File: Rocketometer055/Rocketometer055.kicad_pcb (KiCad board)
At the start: 2 copper layers, 55.9 x 22.9 mm, 58 parts, among them J102 Micro_SD_Card_Det_Hirose_DM3AT, J601 USB_MICROB, J801 JST 2mm, Q650 PMOS, U101 LPC2148, U201 BME280, U301 BNO085, U401 ADXL375, U501 FGPMMOPA6H, U599 FGPMMOPA6H, U701 3.3V, U801 MCP73831, Y101 12MHz, Y301 32kiHz

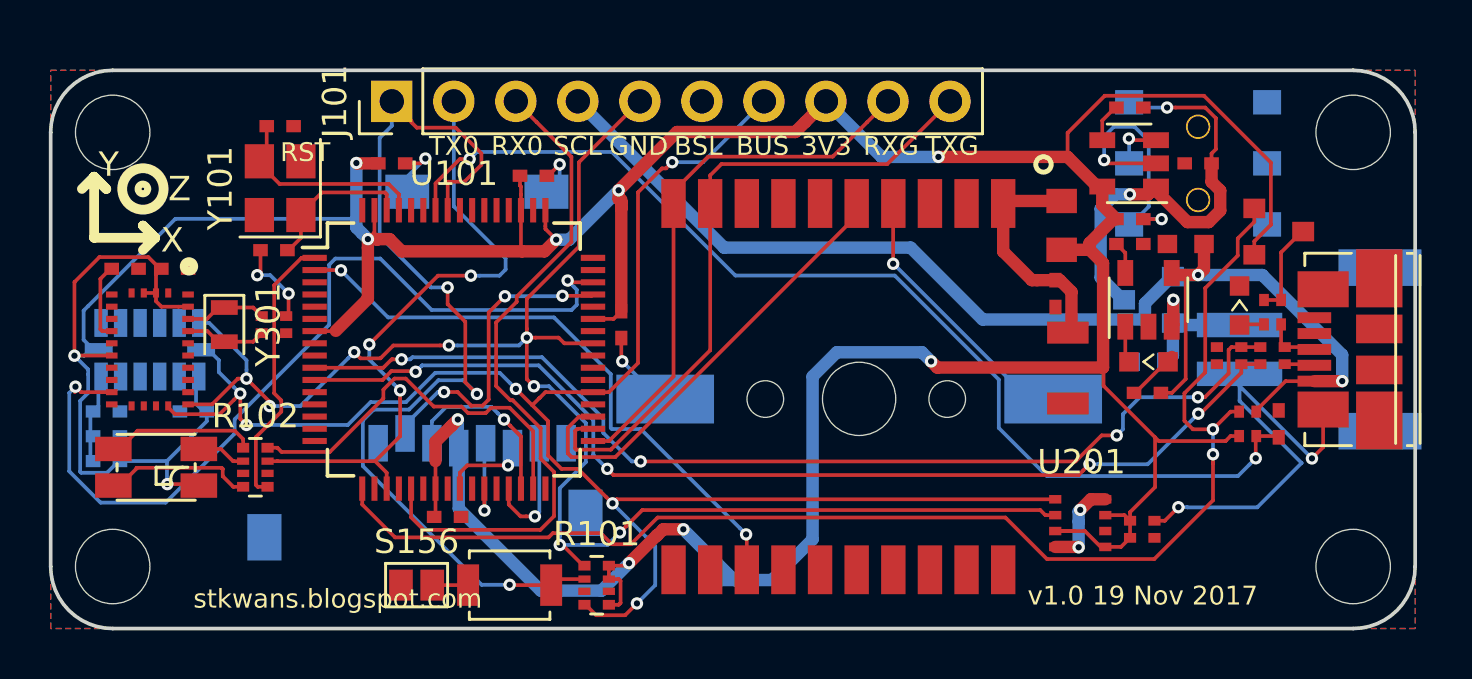
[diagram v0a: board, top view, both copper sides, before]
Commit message: Working on Rocketometer055
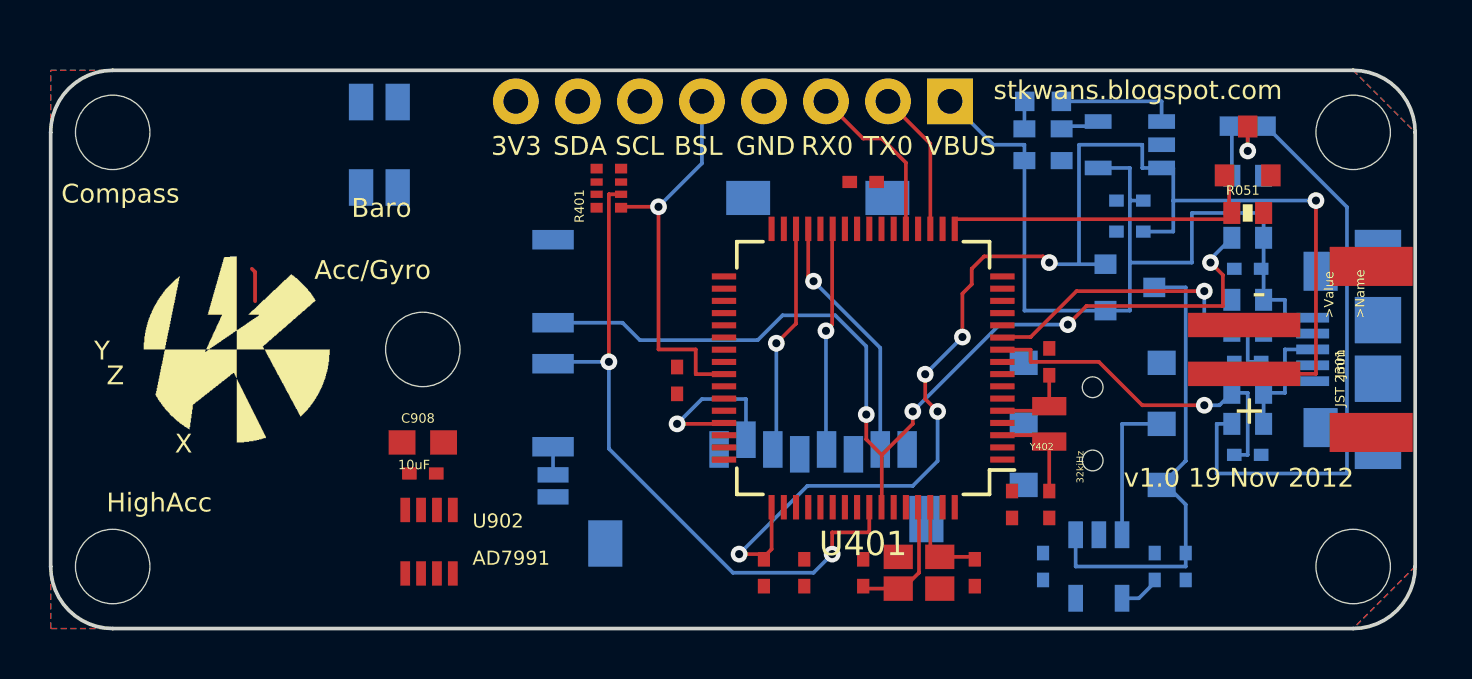
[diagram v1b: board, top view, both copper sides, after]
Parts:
- removed B504: Coin_Cell, KwanSystems:CR1220-2
- removed C123, C406, C704: 1uF, KwanSystems:SMD_0402
- removed C143, C151, C163, C401, C501, C714: 100nF, KwanSystems:SMD_0402
- removed C161, C162: 33pF, KwanSystems:SMD_0402
- removed C206: 100nF, KwanSystems:R_Array_Convex_2x0402
- removed C303, C309: 0.1uF, KwanSystems:SMD_0402
- removed C326, C623: 22pF, KwanSystems:R_Array_Convex_2x0402
- removed C503: 10uF, KwanSystems:SMD_1206
- removed C715: 4.7nF, KwanSystems:SMD_0402
- removed C802, C803: 4.7uF, KwanSystems:SMD_0603
- removed D101: HSMF-C118, KwanSystems:HSMF-C118
- removed D650: BLUE, KwanSystems:D_0603
- removed D801: YELLOW, KwanSystems:D_0603
- removed D802: DCC, KwanSystems:SOT-23
- removed J101: ~, Pin_Headers:Pin_Header_Straight_1x10_Pitch2.54mm
- removed J102: Micro_SD_Card_Det_Hirose_DM3AT, KwanSystems:MICROSD-SOCKET-PP
- removed J601: USB_MICROB, KwanSystems:USB_Micro-B_Molex_47346-0001
- removed J801: JST 2mm, KwanSystems:SPARKFUN_JST_POWER
- removed L501: Ferrite, KwanSystems:SMD_0805
- removed Q650: PMOS, KwanSystems:SOT-23
- removed R101: 10k, KwanSystems:R_Array_Convex_4x0402
- removed R102: 1.5k, KwanSystems:R_Array_Convex_4x0402
- removed R406: 100, KwanSystems:SMD_0402
- removed R611: 22k, KwanSystems:SMD_0402
- removed R623: 33, KwanSystems:R_Array_Convex_2x0402
- removed R650: 1.5k, KwanSystems:R_Array_Convex_2x0402
- removed R651: 10k, KwanSystems:R_Array_Convex_2x0402
- removed R801: 10k, KwanSystems:SMD_0402
- removed R804: 1.5k, KwanSystems:SMD_0402
- removed S156: SOLDERJUMPERNO, Connectors:GS2
- removed S157: SPST, KwanSystems:SW_SPST_B3U-1000P
- removed S701: SPDT, KwanSystems:SWITCH_DPDT_AZY0202
- removed U101: LPC2148, Housings_QFP:LQFP-64_10x10mm_Pitch0.5mm
- removed U501: FGPMMOPA6H, KwanSystems:FGPMMOPA6H
- removed U599: FGPMMOPA6H, KwanSystems:Axis
- removed U701: 3.3V, TO_SOT_Packages_SMD:SOT-23-5
- removed U801: MCP73831, TO_SOT_Packages_SMD:SOT-23-5
- removed Y101: 12MHz, Crystals:Crystal_SMD_Abracon_ABM8G-4pin_3.2x2.5mm
- removed Y301: 32kiHz, Crystals:Crystal_SMD_2012-2pin_2.0x1.2mm
- added C010: 1uF, KwanSystems:SMD_0402, B.Cu at (176.0, 86.9)
- added C020: 22pF, KwanSystems:SMD_0402, B.Cu at (176.0, 90.7)
- added C030: 22pF, KwanSystems:SMD_0402, B.Cu at (176.0, 94.5)
- added C204: 1uF, KwanSystems:SMD_0402, B.Cu at (173.5, 99.1)
- added C214: 100nF, KwanSystems:SMD_0402, B.Cu at (172.2, 99.1)
- added C215: 4.7nF, KwanSystems:SMD_0402, B.Cu at (167.6, 99.1)
- added C301: 4.7uF, KwanSystems:SMD_0402, B.Cu at (171.2, 85.3)
- added C302: 4.7uF, KwanSystems:SMD_0402, B.Cu at (171.2, 84.1)
- added C403: 18pF, KwanSystems:SMD_0402, F.Cu at (167.9, 96.5)
- added C423: 1uF, KwanSystems:SMD_0402, F.Cu at (160.3, 83.3)
- added C443: 100nF, KwanSystems:SMD_0402, F.Cu at (152.7, 91.4)
- added C449: 100nF, KwanSystems:SMD_0402, F.Cu at (156.2, 99.3)
- added C451: 100nF, KwanSystems:SMD_0402, F.Cu at (157.9, 99.3)
- added C461: 33pF, KwanSystems:SMD_0402, F.Cu at (160.3, 99.3)
- added C462: 33pF, KwanSystems:SMD_0402, F.Cu at (164.8, 99.3)
- added C463: 100nF, KwanSystems:SMD_0402, F.Cu at (166.4, 96.5)
- added C907: 100nF, KwanSystems:SMD_0402, F.Cu at (142.2, 95.2)
- added C908: 10uF, 0603-CAP, F.Cu at (142.2, 94.0)
- added D050: BLUE, LED-0603, B.Cu at (176.0, 81.0)
- added D301: YELLOW, LED-0603, B.Cu at (167.6, 80.0)
- added D302: DCC, KwanSystems:SOT-23, B.Cu at (171.2, 87.6)
- added D401: HSMF-C118, HSMF-C118, B.Cu at (140.5, 81.8)
- added J001: USB_MICROB, UB-MC5BR3-SD204-4S, B.Cu at (181.4, 90.2)
- added J301: JST 2mm, JST-2-SMD, F.Cu at (179.6, 90.2)
- added J401: M07, 1X08, F.Cu at (163.8, 80.0)
- added J701: Micro_SD_Card_Det_Hirose_DM3AT, MICROSD-SOCKET-PP, B.Cu at (163.3, 83.6)
- added JP3: STAND-OFFTIGHT, STAND-OFF-TIGHT, F.Cu at (142.2, 90.2)
- added Q050: PMOS, KwanSystems:SOT-23, F.Cu at (176.0, 82.0)
- added R010: 10k, 0402-RES, B.Cu at (176.0, 85.6)
- added R011: 100k, 0402-RES, B.Cu at (176.0, 88.1)
- added R020: 33, 0402-RES, B.Cu at (176.0, 89.4)
- added R030: 33, 0402-RES, B.Cu at (176.0, 91.9)
- added R031: 1.5k, 0402-RES, B.Cu at (176.0, 93.2)
- added R050: 1.5k, 0402-RES, B.Cu at (176.0, 83.1)
- added R051: 10k, 0402-RES, F.Cu at (176.0, 84.6)
- added R301: 10k, 0402-RES, B.Cu at (168.4, 81.8)
- added R302: 1.5k, 0402-RES, B.Cu at (166.9, 81.8)
- added R401: 10k, CRA04, F.Cu at (149.9, 83.6)
- added S201: SPDT, AYZ0202, B.Cu at (169.7, 93.2)
- added S456: SOLDERJUMPERNO, SJ_2S-NO, B.Cu at (147.6, 95.8)
- added S457: SPST, B3U-1000P, B.Cu at (147.6, 92.5)
- added S458: B3U-1000P, B3U-1000P, B.Cu at (147.6, 87.4)
- added U$1: , KWAN_ACC, F.Cu at (134.6, 90.2)
- added U$4: , AXES, F.Cu at (128.3, 94.0)
- added U$5: , KWAN_ACC, B.Cu at (134.6, 90.2)
- added U$6: , OSHW_ACC, B.Cu at (135.9, 98.0)
- added U902: AD7991, SOT-23-8, F.Cu at (142.5, 98.0)
- added Y401: 12MHz, CRYSTAL_SMD_2MM_2_5MM, F.Cu at (162.6, 99.3)
- added Y402: 32kiHz, ABS06, F.Cu at (167.9, 93.2)
- C405: value 100nF -> 18pF; moved to F.Cu
- U201: value BME280 -> 3.3V; footprint KwanSystems:BME280 -> SOT-23-5; moved to B.Cu
- U301: value BNO085 -> MCP73831; footprint KwanSystems:BNO055 -> SOT-23-5; moved to B.Cu
- U401: value ADXL375 -> LPC2148; footprint KwanSystems:ADXL375 -> Housings_QFP:LQFP-64_10x10mm_Pitch0.5mm; moved to F.Cu
- moved U301 41.0 mm to (171.2, 81.8), turned to 270 degrees
- moved C405 38.7 mm to (167.9, 90.7), turned to 270 degrees
- moved U401 29.2 mm to (160.3, 90.9), turned to 180 degrees
- moved U201 1.93 mm to (169.9, 99.1), turned to 0 degrees
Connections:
- C405 pad 1: /HighAcc/VS -> GND
- C405 pad 2: GND -> /RTXC2
- U201 pad 1: GND -> /VIN+
- U201 pad 2: VCC -> GND
- U201 pad 3: /SDA(BSL) -> /PWR_EN
- U201 pad 4: /SCL -> /BYP
- U201 pad 5: GND -> VCC
- U301 pad 1: (no net) -> /N$4
- U301 pad 3: VCC -> /VLIPO
- U301 pad 4: VCC -> /VBUS
- U301 pad 5: GND -> /N$2
- U401 pad 1: VCC -> Net-(U401-Pad1)
- U401 pad 10: (no net) -> /USBD+
- U401 pad 11: (no net) -> /USBD-
- U401 pad 12: GND -> Net-(U401-Pad12)
- U401 pad 13: /SDA(BSL) -> Net-(U401-Pad13)
- U401 pad 14: /SCL -> Net-(U401-Pad14)
- U401 pad 2: GND -> Net-(U401-Pad2)
- U401 pad 3: (no net) -> /RTXC1
- U401 pad 4: GND -> Net-(U401-Pad4)
- U401 pad 5: GND -> /RTXC2
- U401 pad 6: /HighAcc/VS -> GND
- U401 pad 8: (no net) -> Net-(U401-Pad8)
- U401 pad 9: (no net) -> Net-(U401-Pad9)
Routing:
- net VCC: track 192.2 -> 0.00 mm, vias 11 -> 0
- net /SCL: track 71.0 -> 0.00 mm, vias 6 -> 0
- net /SDA(BSL): track 66.6 -> 0.00 mm, vias 8 -> 0
- net /VLIPO: track 0.00 -> 57.1 mm, vias 0 -> 6
- net /USB_SOFTCONNECT: track 53.9 -> 0.00 mm, vias 2 -> 0
- net GND: track 49.2 -> 0.00 mm, vias 12 -> 0
- net /ACCINT: track 35.6 -> 0.00 mm, vias 2 -> 0
- net /USBD+: track 43.9 -> 14.8 mm, vias 4 -> 1
- net /USBD-: track 43.8 -> 14.7 mm, vias 4 -> 1
- net /GPS_TX: track 27.0 -> 0.00 mm
- net /N$6: track 0.00 -> 26.4 mm, vias 0 -> 1
- net /TX0(PWMR): track 26.1 -> 0.00 mm, vias 3 -> 0
- net /PPS: track 24.9 -> 0.00 mm, vias 2 -> 0
- net /GPS_RX: track 22.3 -> 0.00 mm
- net /RX0: track 27.7 -> 7.12 mm
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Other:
- board text added: "+"
- board text added: "-"
- board text added: "Acc/Gyro"
- board text added: "Baro"
- board text added: "Boot"
- board text added: "Compass"
- board text added: "D"
- board text added: "HighAcc"
- board text added: "Reset"
- board text added: "RocketometerMPU6050"
- board text added: "SDA"
- board text added: "St Kwan's Home for"
- board text added: "VBUS"
- board text added: "a division of"
- board text added: "the Terminally ADD"
- board text added: "v1.0 19 Nov 2012"
- board text removed: "BUS"
- board text removed: "RST"
- board text removed: "RXG"
- board text removed: "RocketometerBNO055"
- board text removed: "TXG"
- board text removed: "v1.0 19 Nov 2017"
